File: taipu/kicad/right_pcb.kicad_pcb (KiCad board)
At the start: 2 copper layers, 162.9 x 92.4 mm, 56 parts

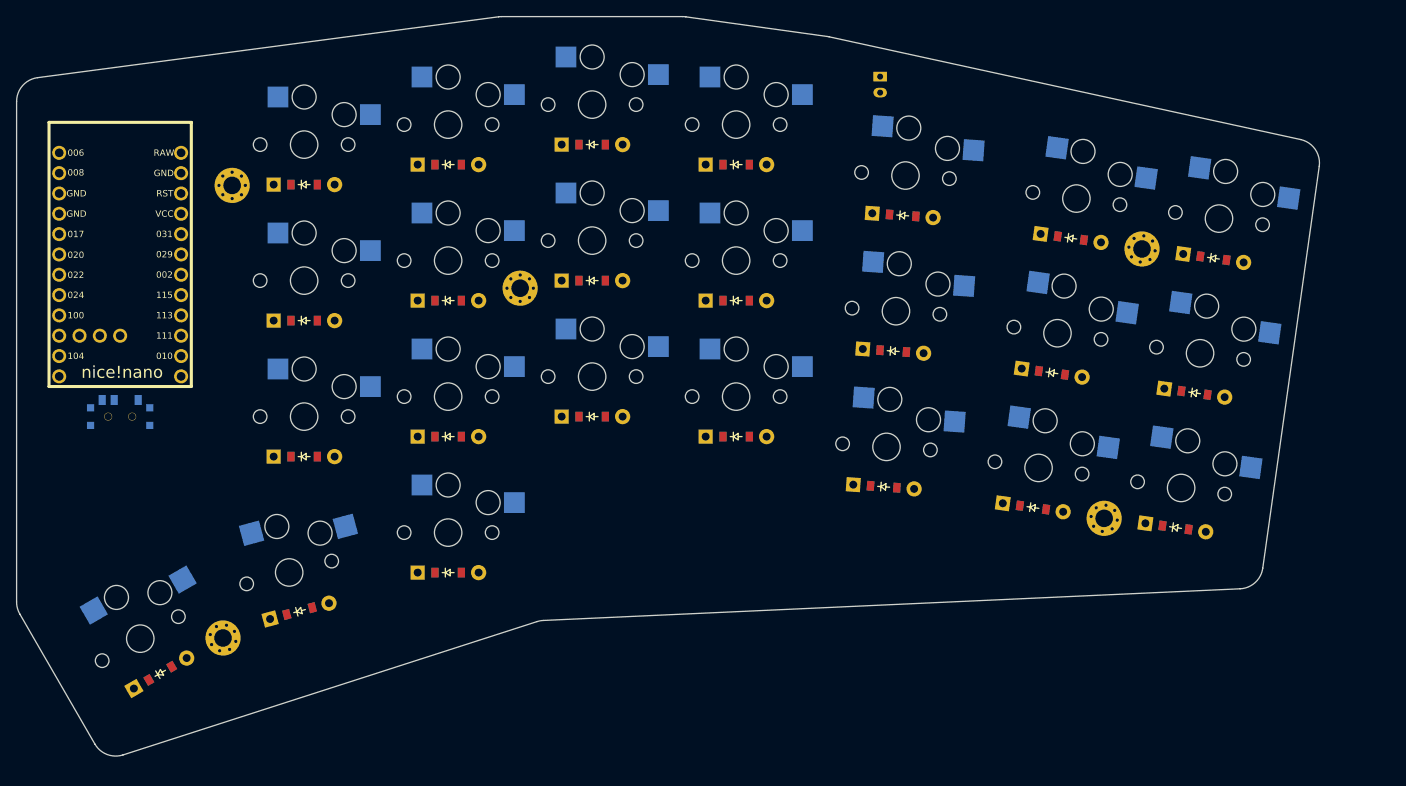
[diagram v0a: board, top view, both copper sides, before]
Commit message: routing
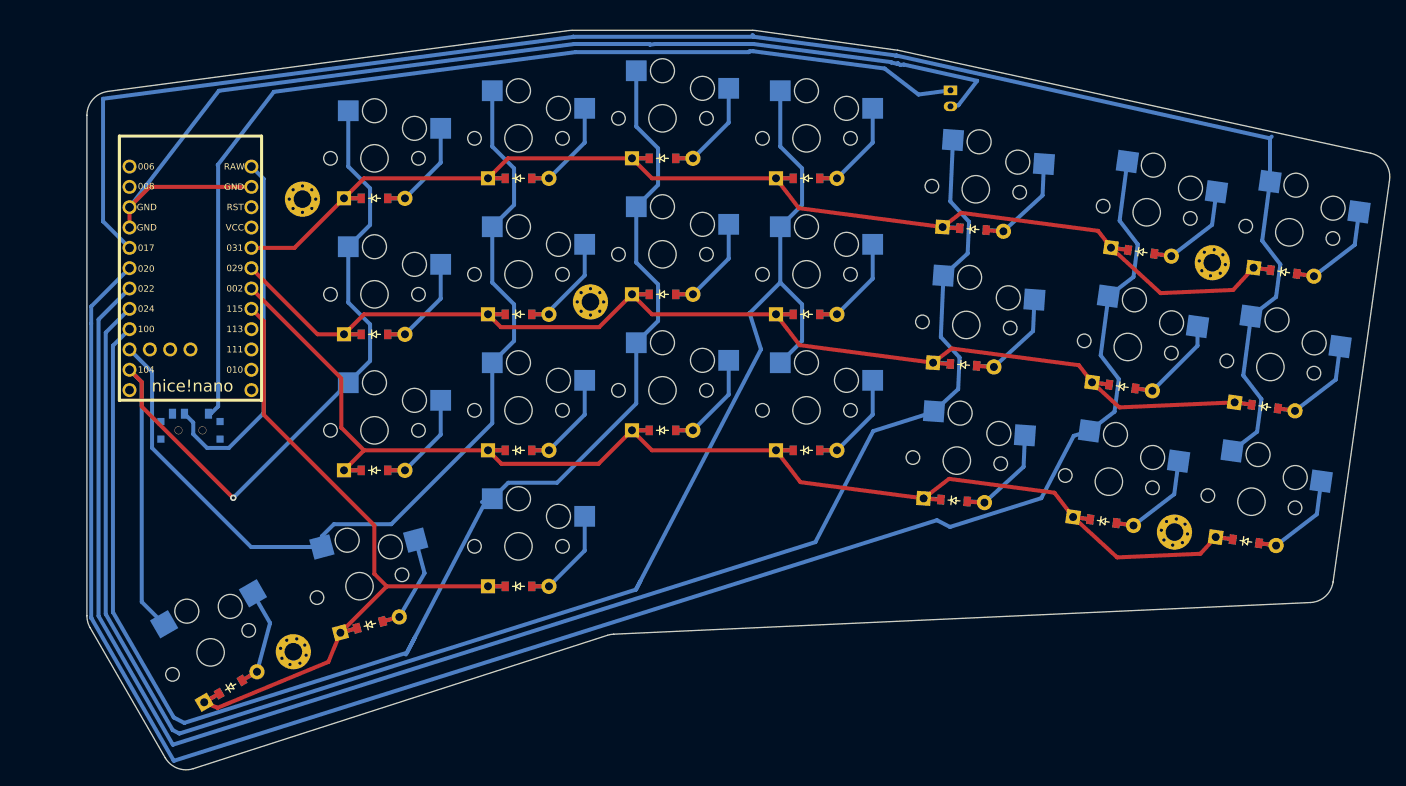
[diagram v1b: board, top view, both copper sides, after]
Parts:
- moved S21 8.96 mm to (276.0, 109.0)
- moved S13 8.96 mm to (312.0, 121.0)
- moved S4 8.96 mm to (367.8, 132.4)
- moved S12 8.96 mm to (330.0, 89.5)
- moved S15 8.96 mm to (312.0, 87.0)
- moved _5 8.96 mm to (265.9, 153.6)
- moved D24 8.96 mm to (258.1, 158.1)
- moved S11 8.96 mm to (330.0, 106.5)
- moved MCU1 8.96 mm to (253.0, 107.0)
- moved D8 8.96 mm to (349.7, 117.8)
- moved D17 8.96 mm to (294.0, 128.5)
- moved S24 8.96 mm to (255.6, 153.7)
- moved S17 8.96 mm to (294.0, 123.5)
- moved D14 8.96 mm to (312.0, 109.0)
- moved S1 8.96 mm to (385.7, 134.9)
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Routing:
- net P020: track 0.00 -> 229.8 mm
- net P017: track 0.00 -> 212.2 mm
- net P022: track 0.00 -> 207.4 mm
- net P024: track 0.00 -> 200.8 mm
- net P002: track 0.00 -> 178.0 mm
- net P100: track 0.00 -> 177.2 mm
- net P031: track 0.00 -> 168.7 mm
- net P029: track 0.00 -> 166.4 mm
- net GND: track 0.00 -> 137.8 mm
- net pos: track 0.00 -> 130.0 mm
- net P011: track 0.00 -> 114.4 mm
- net P104: track 0.00 -> 113.9 mm, vias 0 -> 1
- net P115: track 0.00 -> 96.3 mm
- net RAW: track 0.00 -> 45.8 mm
- net mirror_pinky_home: track 0.00 -> 14.9 mm
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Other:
- net class Default removed
